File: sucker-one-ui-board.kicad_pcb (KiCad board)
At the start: 2 copper layers, 36.4 x 48.3 mm, 32 parts, among them J1 52271-1079, Q1 BSS138, SW1 LIFT, SW2 LOW, SW3 REVERSE, SW4 TRIGGER, SW5 DROP, SW6 HIGH, U1 WS2812-2020, U10 WS2812-2020, U11 WS2812-2020, U12 WS2812-2020, U2 WS2812-2020, U3 WS2812-2020, U4 WS2812-2020, U5 WS2812-2020, U6 WS2812-2020, U7 WS2812-2020, U8 WS2812-2020, U9 WS2812-2020

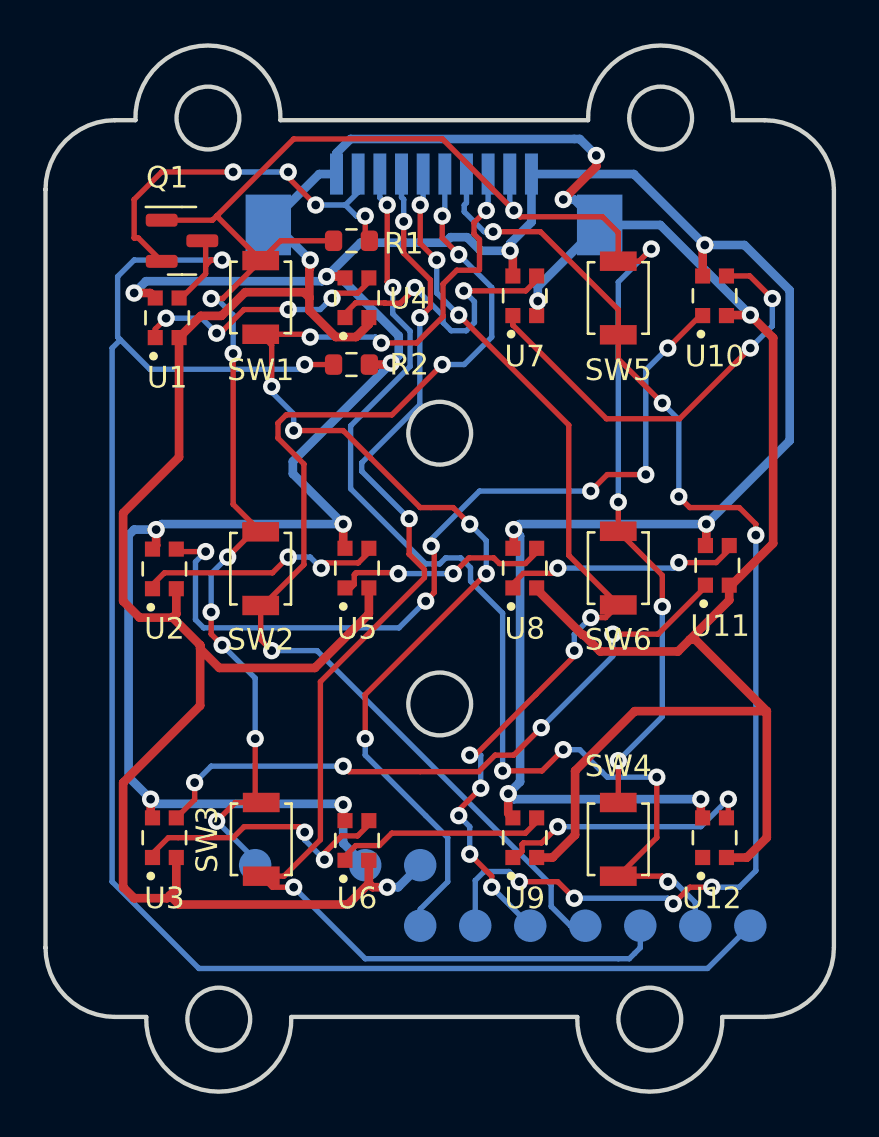
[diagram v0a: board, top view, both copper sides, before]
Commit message: Update design and generate gerbers
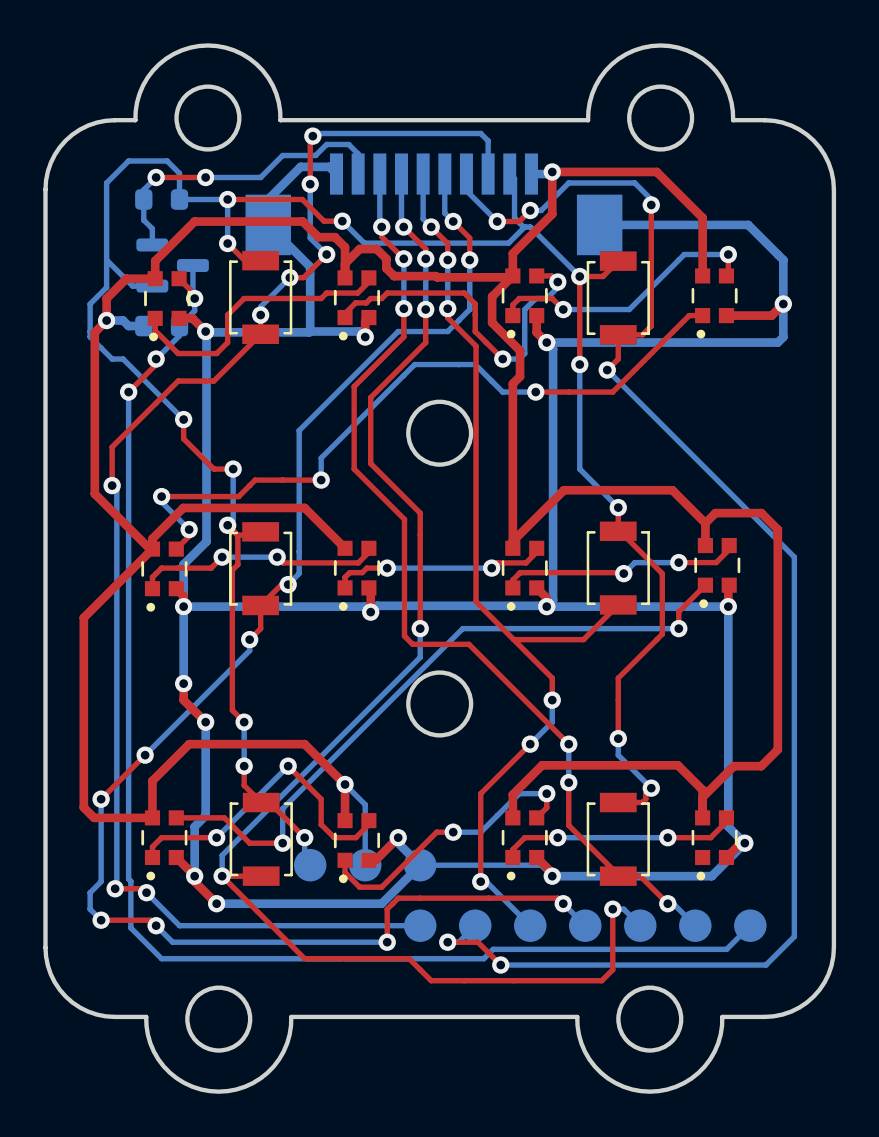
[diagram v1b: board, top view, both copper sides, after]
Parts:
- Q1, R1, R2: moved to B.Cu
- moved R1 8.97 mm to (69.1, 69.6), turned to 0 degrees
- moved R2 8.94 mm to (69.1, 75.4), turned to 180 degrees
- moved TP10 2.54 mm to (75.9, 100.3)
- moved Q1 1.22 mm to (69.6, 72.6)
- moved U1 0.89 mm to (69.3, 74.2)
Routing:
- net LED_DATA: track 80.1 -> 63.0 mm, vias 2 -> 3
- net LOW_BTN: track 52.5 -> 68.9 mm, vias 4 -> 10
- net +5V: track 144.2 -> 158.4 mm, vias 13 -> 3
- net DROP_BTN: track 57.1 -> 68.6 mm, vias 8 -> 6
- net LIFT_BTN: track 55.6 -> 65.3 mm
- net TRIGGER_BTN: track 52.0 -> 44.9 mm
- net Net-(U10-Pad3): track 19.8 -> 12.9 mm
- net +3V3: track 98.4 -> 105.1 mm, vias 12 -> 14
- net REVERSE_BTN: track 59.5 -> 65.1 mm, vias 4 -> 6
- net DO_DROP: track 38.7 -> 33.3 mm, vias 6 -> 4
- net GND: track 167.5 -> 162.8 mm, vias 6 -> 15
- net DO_REV: track 9.87 -> 13.3 mm, vias 0 -> 2
- net Net-(J1-Pad9): track 18.6 -> 15.4 mm, vias 4 -> 2
- net DO_LIFT: track 13.3 -> 16.3 mm
- net Net-(U3-Pad1): track 12.6 -> 14.5 mm
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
